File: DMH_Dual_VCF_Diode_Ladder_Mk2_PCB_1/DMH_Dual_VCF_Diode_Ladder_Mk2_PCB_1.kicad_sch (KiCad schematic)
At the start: 0 parts

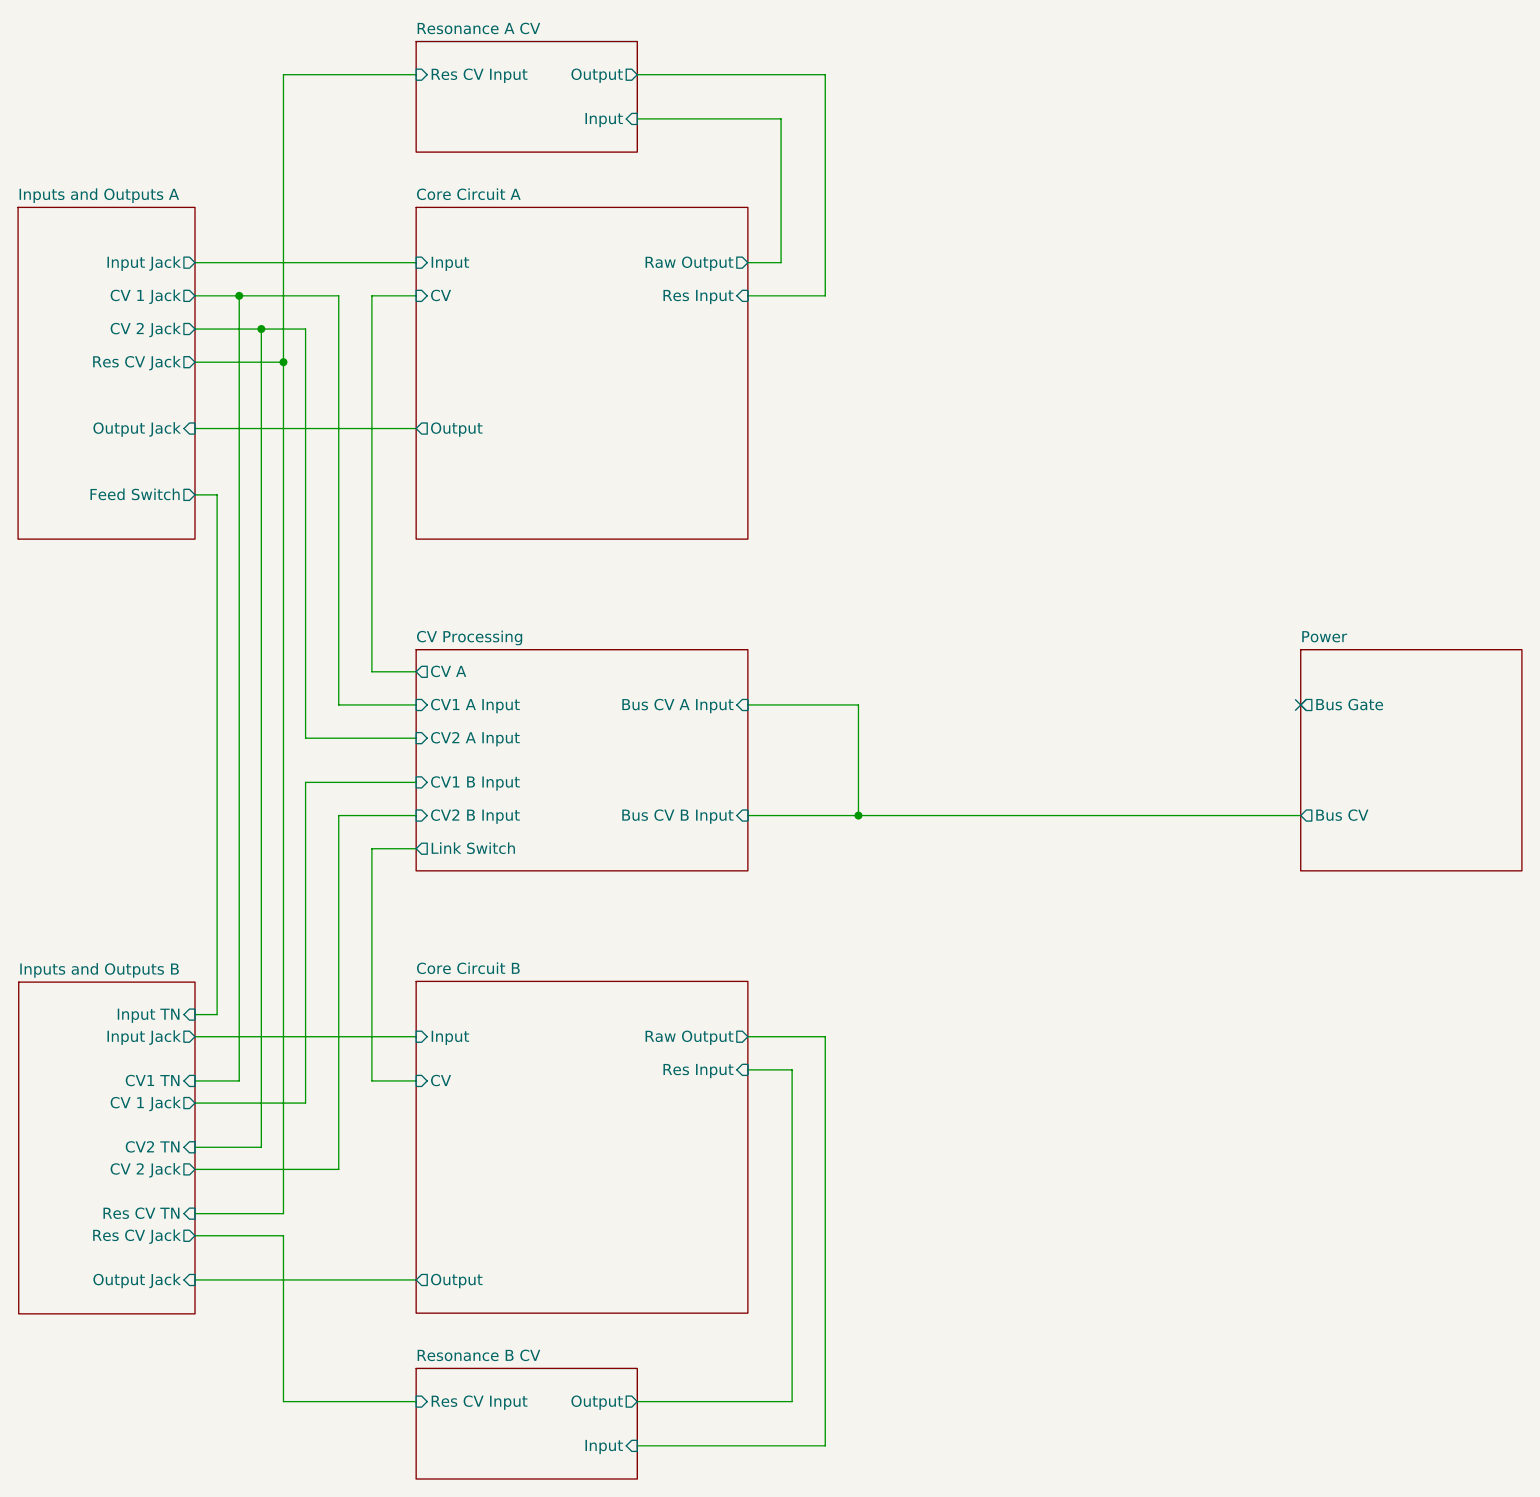
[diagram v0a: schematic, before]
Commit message: Added CV3 and Drive CV to I/O pages
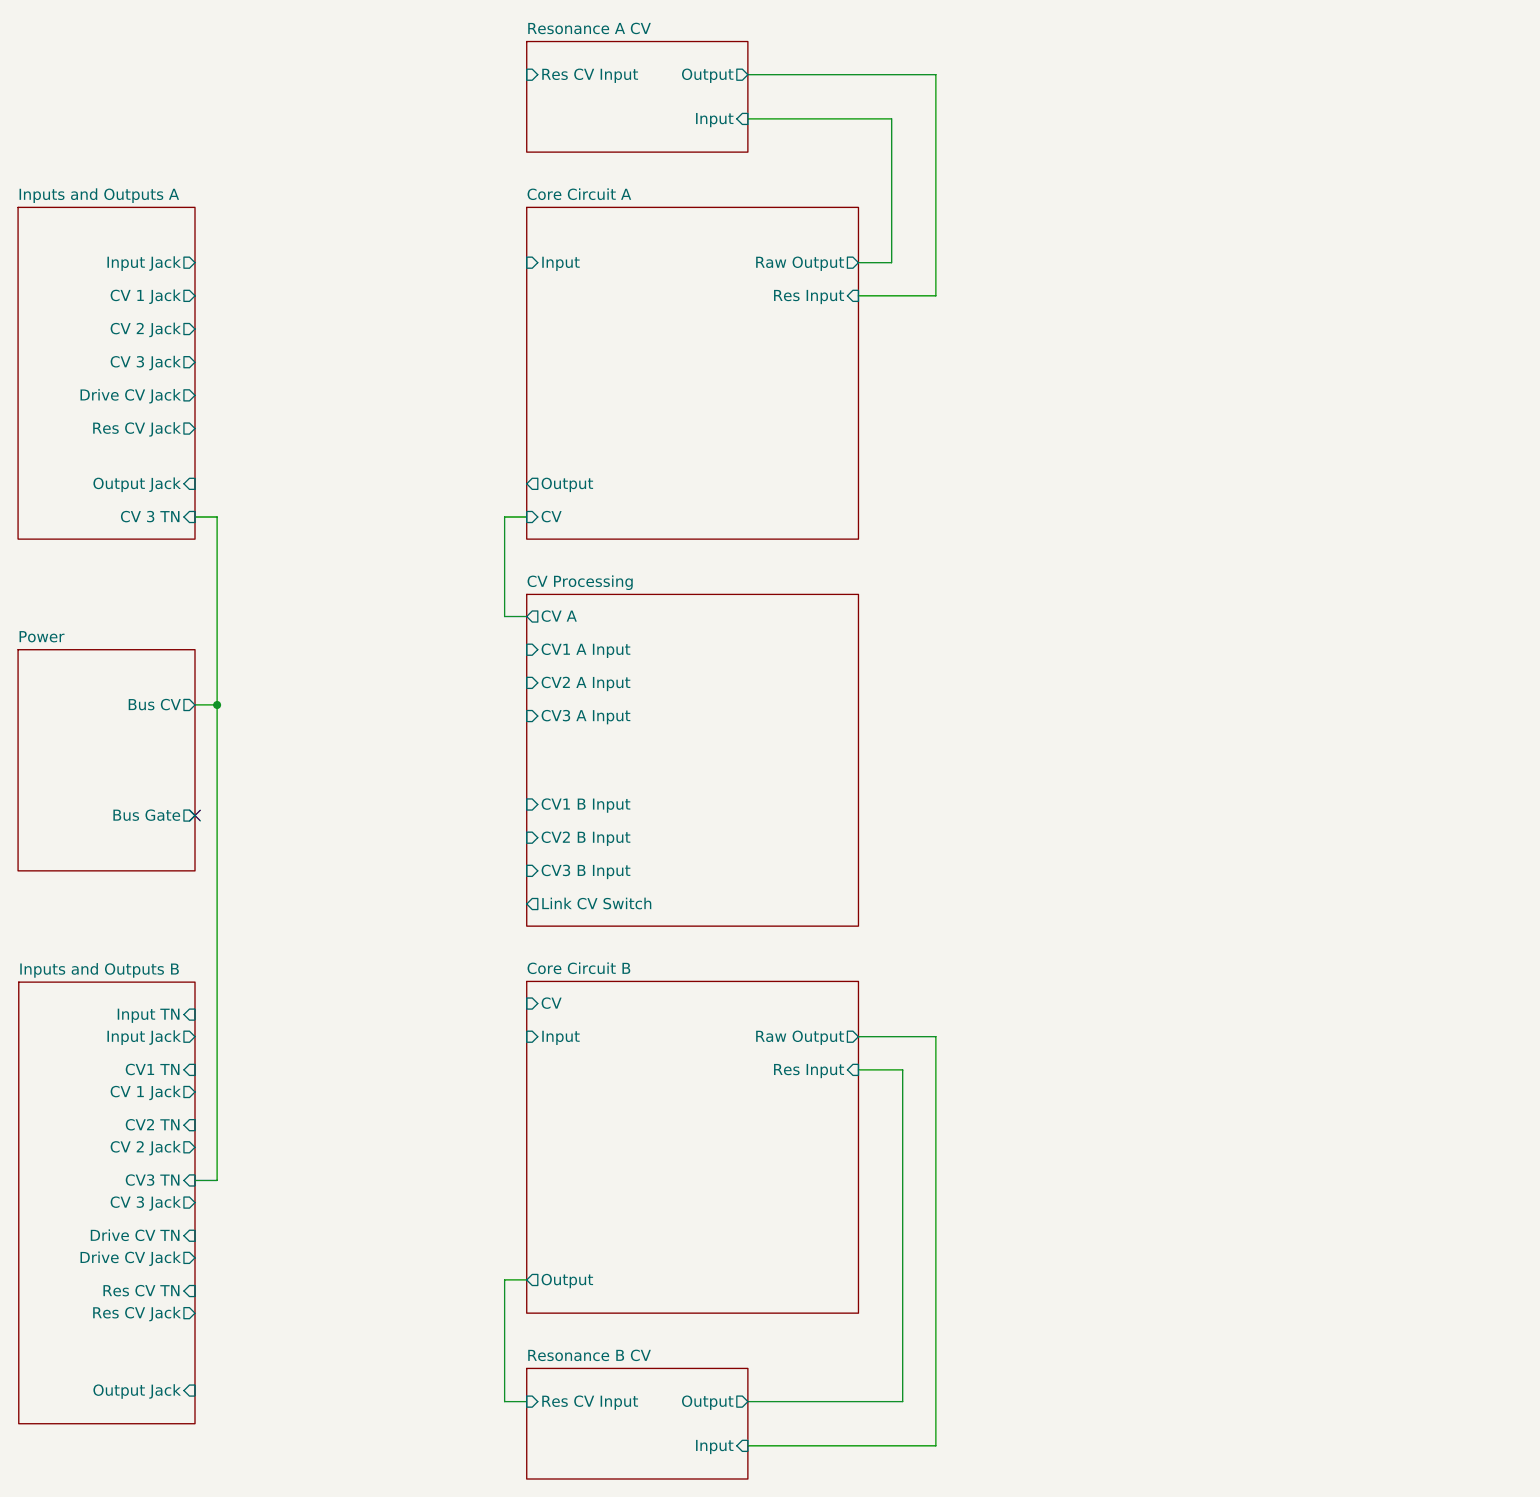
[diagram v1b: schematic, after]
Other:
- sheet CV Processing ports: added CV3 A Input, CV3 B Input, Link CV Switch; removed Bus CV A Input, Bus CV B Input, Link Switch
- sheet Inputs and Outputs A ports: added CV 3 Jack, CV 3 TN, Drive CV Jack; removed Feed Switch
- sheet Inputs and Outputs B ports: added CV 3 Jack, CV3 TN, Drive CV Jack, Drive CV TN; removed none
